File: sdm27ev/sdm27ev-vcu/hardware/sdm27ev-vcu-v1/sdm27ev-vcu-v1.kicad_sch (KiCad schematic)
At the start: 3 parts, among them J1 6437288-1, J2 6437288-1, U1 ESP32-P4

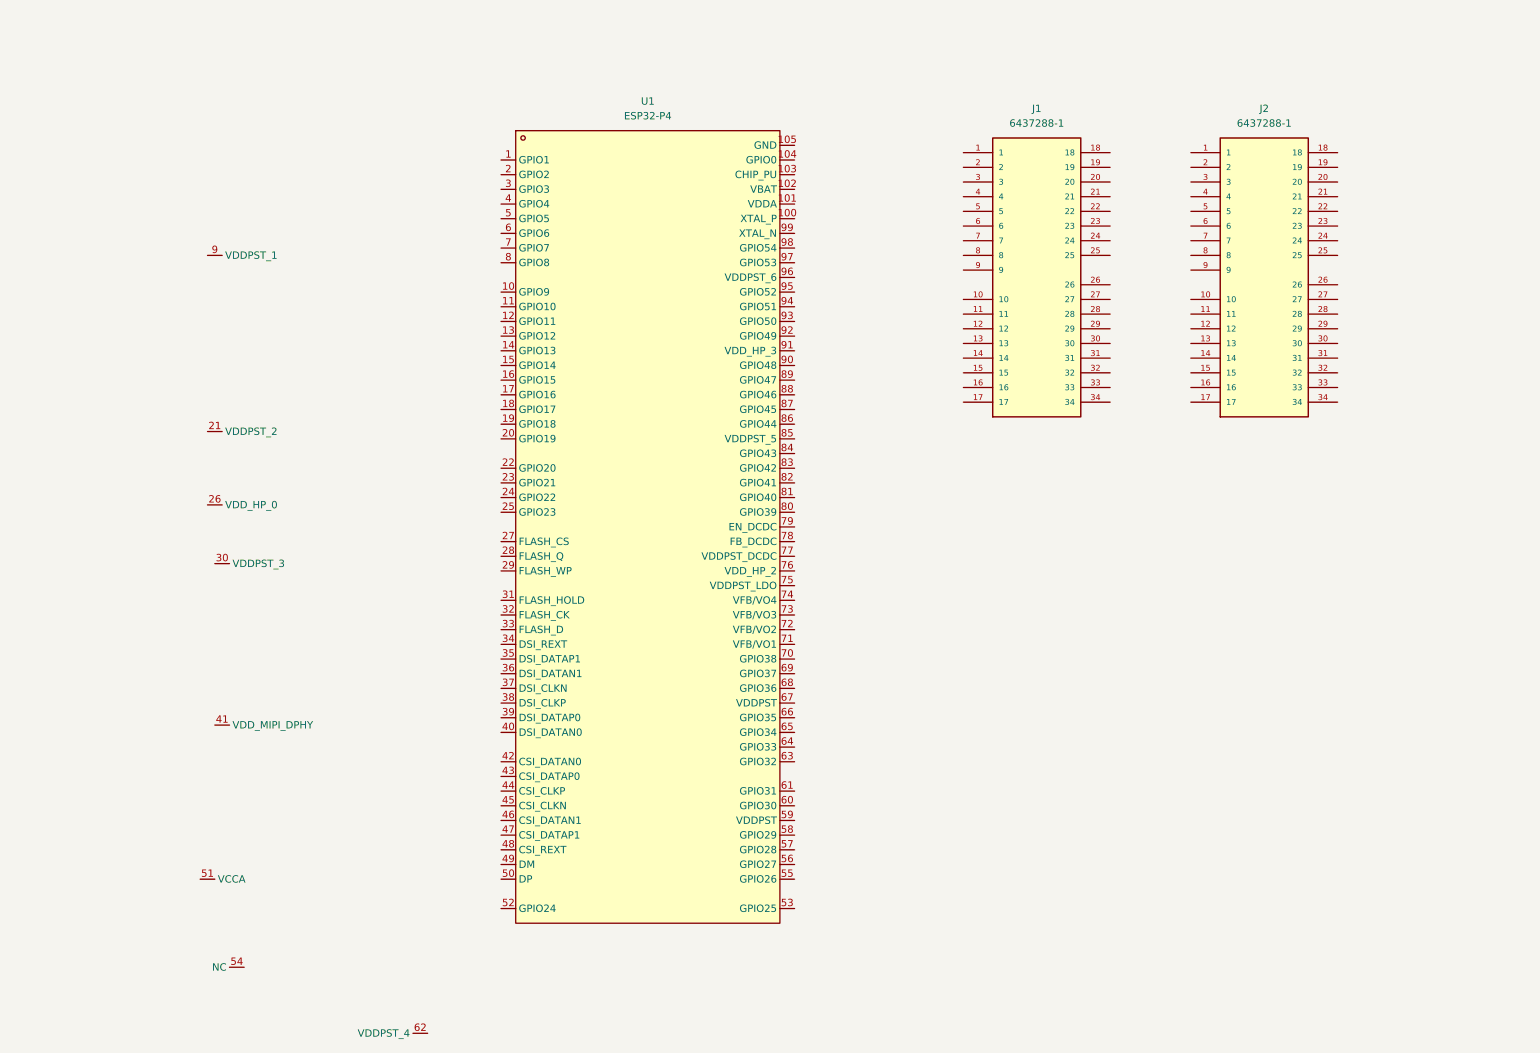
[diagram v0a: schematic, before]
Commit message: VCU sch updates
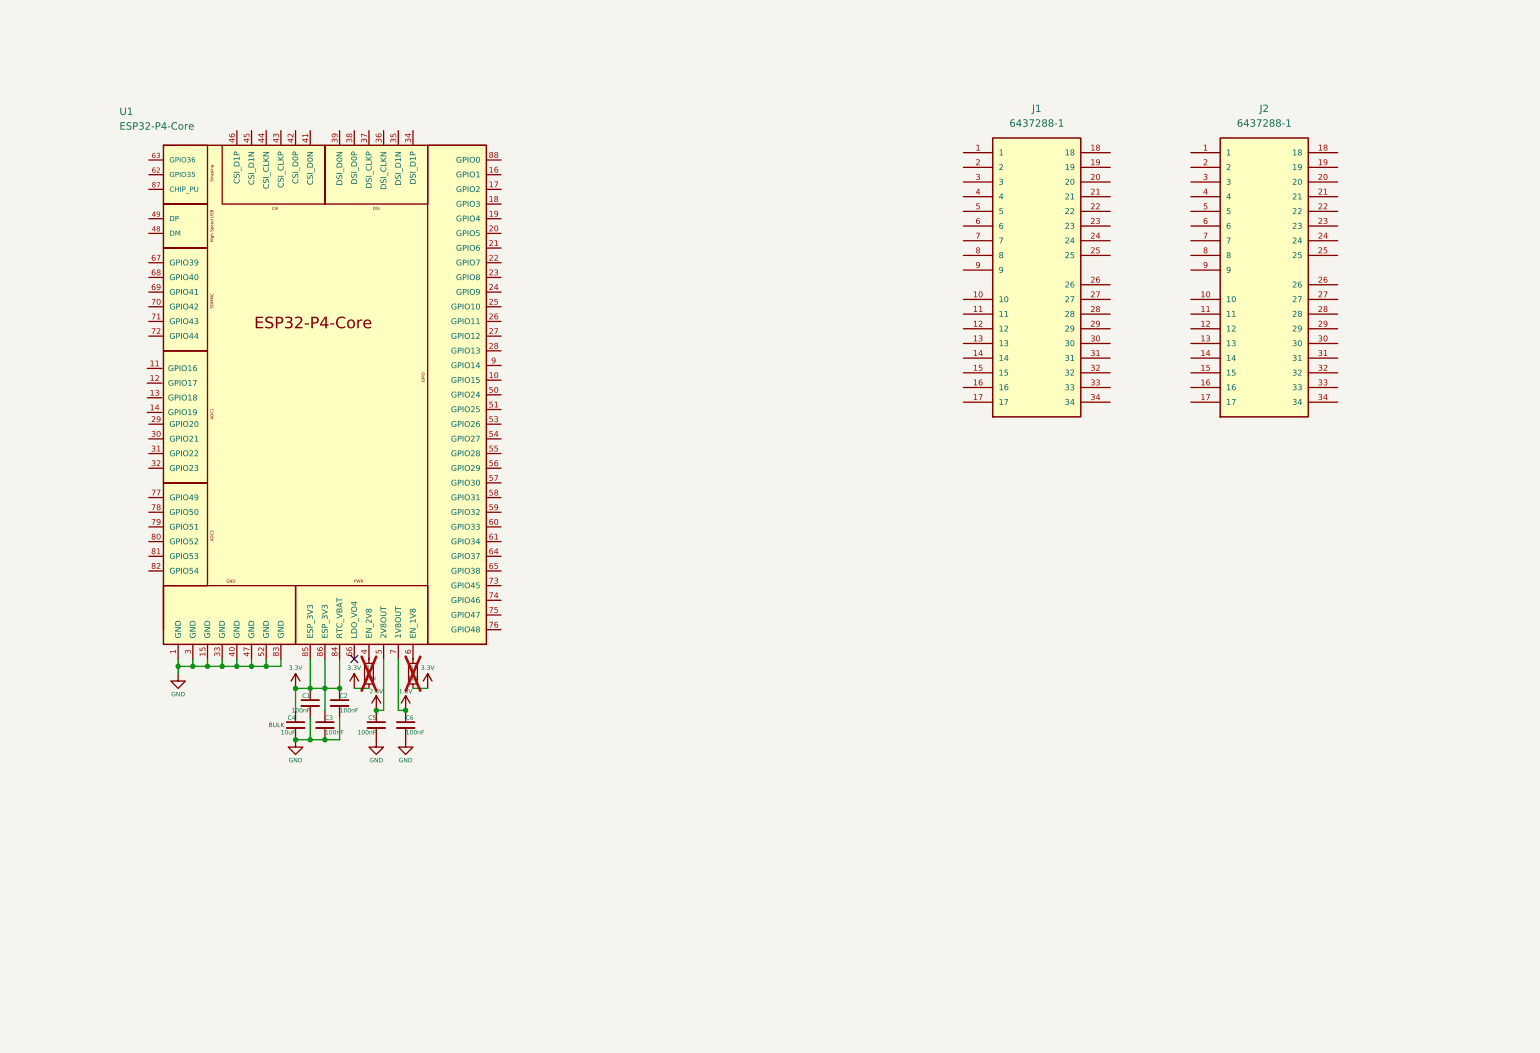
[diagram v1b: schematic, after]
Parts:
- removed U1: ESP32-P4, SDM27 EV VCU:QFN-104_L10.0-W10.0-P0.35-TL-EP7.5, symbol EV VCU:ESP32-P4
- added C1, C2, C3, C5, C6: 100nF, Capacitor_SMD:C_0603_1608Metric, symbol Device:C_Small
- added C4: 10uF, Capacitor_SMD:C_0603_1608Metric, symbol Device:C_Small
- added R1, R2: 10k, Resistor_SMD:R_0603_1608Metric, symbol Device:R_Small
- added U1: ESP32-P4-Core, symbol SDM_EV:ESP32-P4-Core
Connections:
- new net: R2.1, U1.4 (EN_2V8)
- new net: R1.1, U1.6 (EN_1V8)
- new net 1.8V: C6.1, U1.7 (1V8OUT)
- new net 2.8V: C5.1, U1.5 (2V8OUT)
- new net 3.3V: C1.1, C2.1, C3.1, C4.1, R1.2, R2.2, U1.84 (RTC_VBAT), U1.85 (ESP_3V3), U1.86 (ESP_3V3)
- new net GND: C1.2, C2.2, C3.2, C4.2, C5.2, C6.2, U1.1 (GND), U1.15 (GND), U1.3 (GND), U1.33 (GND), U1.40 (GND), U1.47 (GND), U1.52 (GND), U1.83 (GND)
- no-connect marks 0 -> 1
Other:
- note added: "BULK"

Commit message: more VCU updates
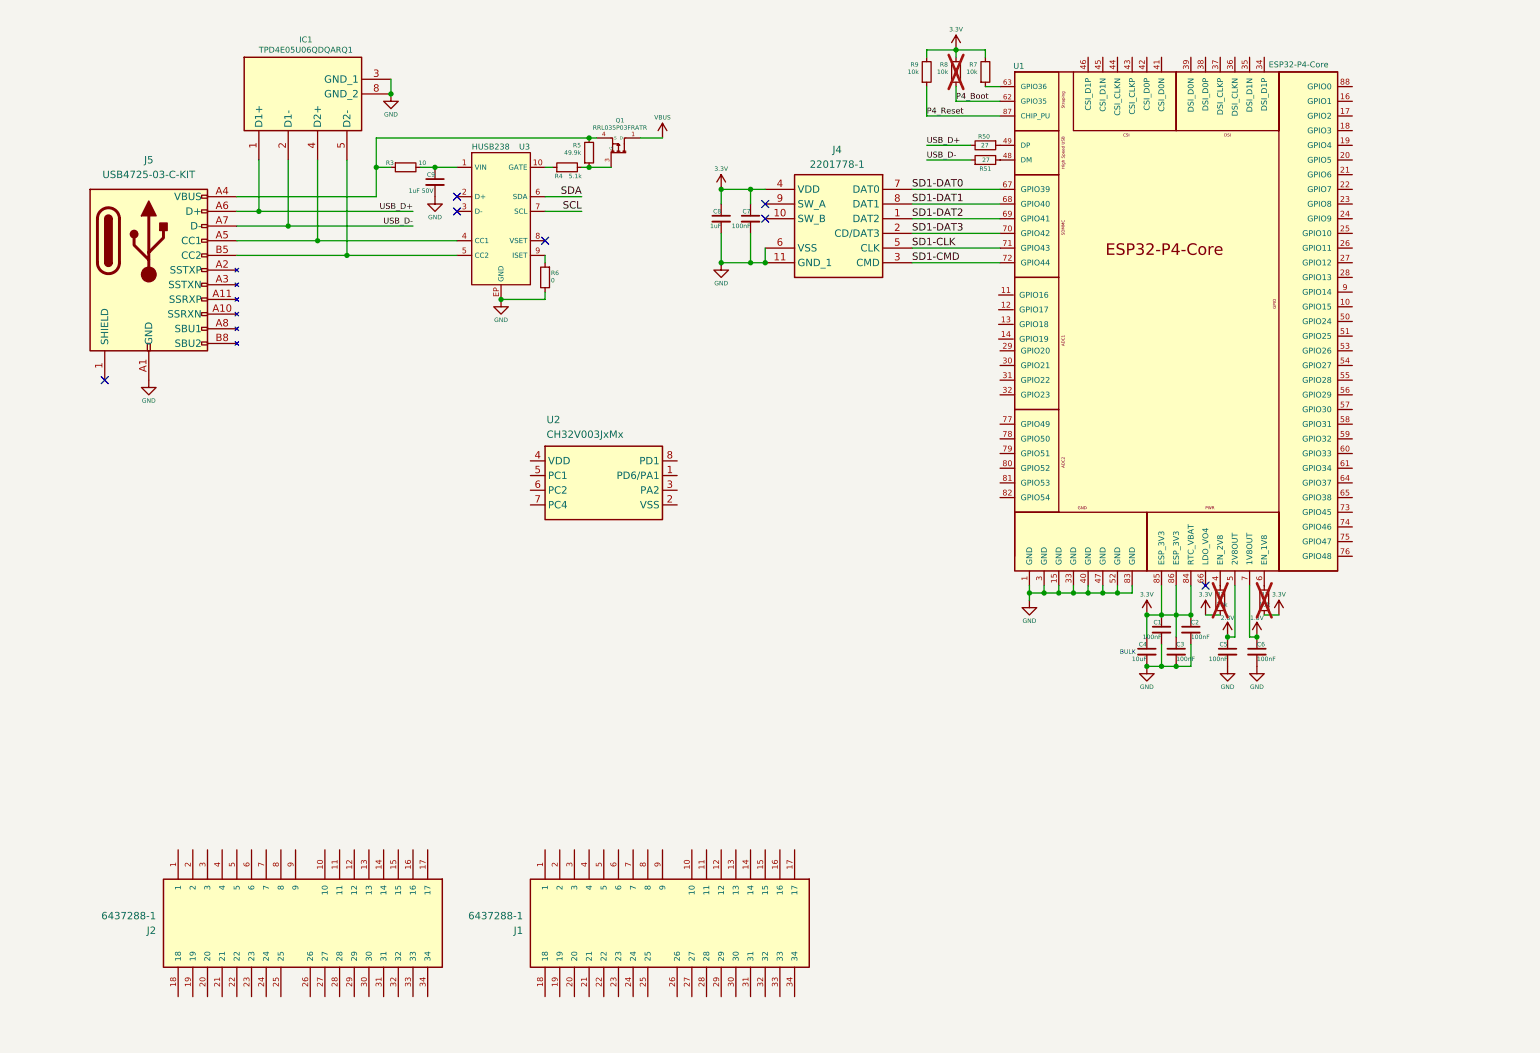
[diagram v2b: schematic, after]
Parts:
- added C7: 100nF, Capacitor_SMD:C_0603_1608Metric, symbol Device:C_Small
- added C8: 1uF, Capacitor_SMD:C_0603_1608Metric, symbol Device:C_Small
- added C9: 1uF 50V, Capacitor_SMD:C_0603_1608Metric, symbol Device:C_Small
- added IC1: TPD4E05U06QDQARQ1, DQA(R-PUSON-N10), symbol SDM_EV:TPD4E05U06QDQARQ1
- added J4: 2201778-1, 22017781, symbol SDM_EV:2201778-1
- added J5: USB4725-03-C-KIT, SDM_Misc:GCT_USB4730-GF-A_REVA, symbol SDM_MISC:USB4725-03-C-KIT
- added Q1: RRL035P03FRATR, RRL035P03FRATR, symbol SDM_EV:RRL035P03FRATR
- added R3: 10, Resistor_SMD:R_0603_1608Metric, symbol Device:R_Small
- added R4: 5.1k, Resistor_SMD:R_0603_1608Metric, symbol Device:R_Small
- added R5: 49.9k, Resistor_SMD:R_0603_1608Metric, symbol Device:R_Small
- added R50, R51: 27, Resistor_SMD:R_0402_1005Metric, symbol Device:R_Small
- added R6: 0, Resistor_SMD:R_0603_1608Metric, symbol Device:R_Small
- added R7, R8, R9: 10k, Resistor_SMD:R_0603_1608Metric, symbol Device:R_Small
- added U2: CH32V003JxMx, Package_SO:JEITA_SOIC-8_3.9x4.9mm_P1.27mm, symbol MCU_WCH_RiscV:CH32V003JxMx
- added U3: HUSB238, symbol SDM_EV:HUSB238
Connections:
- net 3.3V: now also C7.1, C8.1, J4.4 (VDD), R7.2, R8.2, R9.2
- net GND: now also C7.2, C8.2, C9.2, IC1.3 (GND_1), IC1.8 (GND_2), J4.11 (GND_1), J4.12 (GND_2), J4.13 (GND_3), J4.14 (GND_4), J4.15 (GND_5), J4.16 (GND_6), J4.6 (VSS), J5.A1 (GND), R6.2, U3.EP (GND)
- net at U1.48 (DM): now also R51.2
- net at U1.49 (DP): now also R50.1
- net P4_Boot: now reaches U1.62 (GPIO35)
- net P4_Boot: now also R8.1
- net at U1.63 (GPIO36): now also R7.1
- net SD1-DAT0: now reaches U1.67 (GPIO39)
- net SD1-DAT0: now also J4.7 (DAT0)
- net SD1-DAT1: now reaches U1.68 (GPIO40)
- net SD1-DAT1: now also J4.8 (DAT1)
- net SD1-DAT2: now reaches U1.69 (GPIO41)
- net SD1-DAT2: now also J4.1 (DAT2)
- net SD1-DAT3: now reaches U1.70 (GPIO42)
- net SD1-DAT3: now also J4.2 (CD/DAT3)
- net SD1-CLK: now reaches U1.71 (GPIO43)
- net SD1-CLK: now also J4.5 (CLK)
- net SD1-CMD: now reaches U1.72 (GPIO44)
- net SD1-CMD: now also J4.3 (CMD)
- net P4_Reset: now reaches U1.87 (CHIP_PU)
- net P4_Reset: now also R9.1
- new net: C9.1, R3.2, U3.1 (VIN)
- new net: R4.1, U3.10 (GATE)
- new net: IC1.4 (D2+), J5.A5 (CC1), U3.4 (CC1)
- new net: IC1.5 (D2-), J5.B5 (CC2), U3.5 (CC2)
- new net: R6.1, U3.9 (ISET)
- new net: Q1.3 (G), R4.2, R5.1
- new net: J5.A4 (VBUS), Q1.4 (S), R3.1, R5.2
- new net: IC1.10 (NC_3), IC1.6 (NC_4), IC1.7 (NC_1), IC1.9 (NC_2)
- new net SCL: U3.7 (SCL)
- new net SDA: U3.6 (SDA)
- new net USB_D+: IC1.1 (D1+), J5.A6 (D+), J5.B6 (D+), R50.2
- new net USB_D-: IC1.2 (D1-), J5.A7 (D-), J5.B7 (D-), R51.1
- new net VBUS: Q1.1 (D), Q1.2 (D_2), Q1.5 (D_3), Q1.6 (D_4)
- no-connect marks 1 -> 7
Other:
- moved on the sheet: C1, C2, C3, C4, C5, C6, J1, J2, R1, R2, U1

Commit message: Final VCU updates for the night
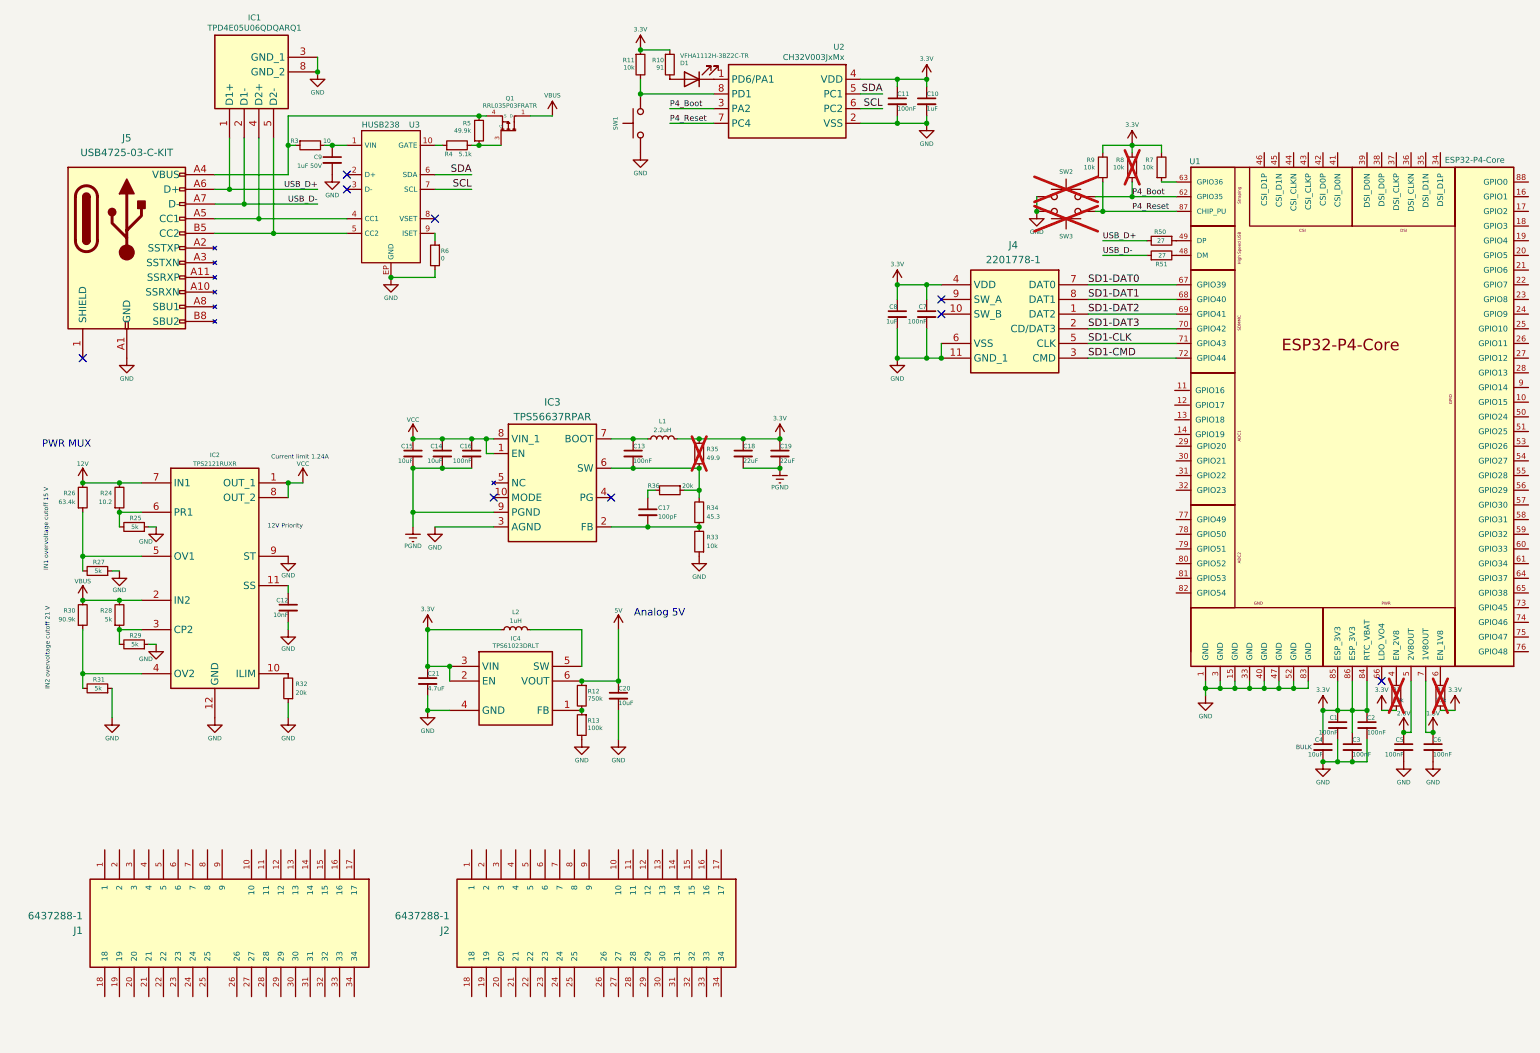
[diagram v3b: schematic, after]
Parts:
- added C10: 1uF, Capacitor_SMD:C_0603_1608Metric, symbol Device:C_Small
- added C11, C13, C16: 100nF, Capacitor_SMD:C_0603_1608Metric, symbol Device:C_Small
- added C12: 10nF, Capacitor_SMD:C_0603_1608Metric, symbol Device:C_Small
- added C14, C15, C20: 10uF, Capacitor_SMD:C_0603_1608Metric, symbol Device:C_Small
- added C17: 100pF, Capacitor_SMD:C_0603_1608Metric, symbol Device:C_Small
- added C18, C19: 22uF, Capacitor_SMD:C_0603_1608Metric, symbol Device:C_Small
- added C21: 4.7uF, Capacitor_SMD:C_0603_1608Metric, symbol Device:C_Small
- added D1: VFHA1112H-3BZ2C-TR, LED_SMD:LED_0805_2012Metric, symbol Device:LED
- added IC2: TPS2121RUXR, SDM_Misc:TPS2121RUXR, symbol SDM_MISC:TPS2121RUXR
- added IC3: TPS56637RPAR, TPS56637RPAR, symbol SDM_EV:TPS56637RPAR
- added IC4: TPS61023DRLT, SOTFL50P160X60-6N, symbol SDM_EV:TPS61023DRLT
- added L1: 2.2uH, Inductor_SMD:L_7.3x7.3_H3.5, symbol Device:L_Small
- added L2: 1uH, Inductor_SMD:L_Changjiang_FTC404010S, symbol Device:L_Small
- added R10: 91, Resistor_SMD:R_0603_1608Metric, symbol Device:R_Small
- added R11: 10k, Resistor_SMD:R_0603_1608Metric, symbol Device:R_Small
- added R12: 750k, Resistor_SMD:R_0603_1608Metric, symbol Device:R_Small
- added R13: 100k, Resistor_SMD:R_0603_1608Metric, symbol Device:R_Small
- added R24: 10.2, Resistor_SMD:R_0402_1005Metric, symbol Device:R_Small
- added R25, R27, R28, R29, R31: 5k, Resistor_SMD:R_0402_1005Metric, symbol Device:R_Small
- added R26: 63.4k, Resistor_SMD:R_0402_1005Metric, symbol Device:R_Small
- added R30: 90.9k, Resistor_SMD:R_0402_1005Metric, symbol Device:R_Small
- added R32, R36: 20k, Resistor_SMD:R_0402_1005Metric, symbol Device:R_Small
- added R33: 10k, Resistor_SMD:R_0402_1005Metric, symbol Device:R_Small
- added R34: 45.3, Resistor_SMD:R_0402_1005Metric, symbol Device:R_Small
- added R35: 49.9, Resistor_SMD:R_0402_1005Metric, symbol Device:R_Small
- added SW1, SW2, SW3: SW_Push, Button_Switch_SMD:SW_SPST_CK_KXT3, symbol Switch:SW_Push
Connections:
- net 3.3V: now also U2.4 (VDD), C10.1, C11.1, C18.1, C19.1, C21.1, IC4.2 (EN), IC4.3 (VIN), L1.2, L2.1, R10.1, R11.1, R35.2
- net GND: now also U2.2 (VSS), C10.2, C11.2, C12.2, C20.2, C21.2, IC2.12 (GND), IC2.9 (ST), IC3.3 (AGND), IC4.4 (GND), R13.2, R25.1, R27.1, R29.1, R31.1, R32.1, R33.1, SW1.1, SW2.1, SW3.2
- net P4_Boot: now also U2.3 (PA2), SW2.2
- net P4_Reset: now also U2.7 (PC4), SW3.1
- net SCL: now also U2.6 (PC2)
- net SDA: now also U2.5 (PC1)
- net VBUS: now also IC2.2 (IN2), R28.2, R30.2
- net at U2.1 (PD6/PA1): now also D1.1 (K)
- net at U2.8 (PD1): now also R11.2, SW1.2
- new net: C13.2, IC3.6 (SW), R34.2, R35.1, R36.1
- new net: C17.1, R36.2
- new net: IC2.5 (OV1), R26.1, R27.2
- new net: IC2.6 (PR1), R24.1, R25.2
- new net: IC4.1 (FB), R12.2, R13.1
- new net: D1.2 (A), R10.2
- new net: C17.2, IC3.2 (FB), R33.2, R34.1
- new net: IC2.10 (ILIM), R32.2
- new net: C12.1, IC2.11 (SS)
- new net: IC2.3 (CP2), R28.1, R29.2
- new net: IC2.4 (OV2), R30.1, R31.2
- new net: C13.1, IC3.7 (BOOT), L1.1
- new net: IC4.5 (SW), L2.2
- new net 12V: IC2.7 (IN1), R24.2, R26.2
- new net 5V: C20.1, IC4.6 (VOUT), R12.1
- new net PGND: C14.2, C15.2, C16.2, C18.2, C19.2, IC3.9 (PGND)
- new net VCC: C14.1, C15.1, C16.1, IC2.1 (OUT_1), IC2.8 (OUT_2), IC3.1 (EN), IC3.11 (VIN_2), IC3.12 (VIN_3), IC3.13 (VIN_4), IC3.8 (VIN_1)
- no-connect marks 7 -> 9
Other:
- note added: "12V Priority"
- note added: "Analog 5V"
- note added: "Current limit 1.24A"
- note added: "IN1 overvoltage cutoff 15 V"
- note added: "IN2 overvoltage cutoff 21 V"
- note added: "PWR MUX"
- moved on the sheet: C1, C2, C3, C4, C5, C6, C7, C8, C9, IC1, J1, J2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
